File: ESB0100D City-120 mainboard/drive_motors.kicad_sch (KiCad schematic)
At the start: 47 parts, among them J1 Conn_01x02, J4 Conn_01x02, Q1 NPN, Q10 IRFZ44N, Q11 SPB18P06P, Q12 IRFZ44N, Q13 NPN, Q14 NPN, Q15 NPN, Q16 NPN, Q17 SPB18P06P, Q18 IRFZ44N, Q19 SPB18P06P, Q2 NPN, Q20 IRFZ44N, Q21 NPN, Q22 NPN, Q3 SPB18P06P, U10 74LS157, U11 74LS157, U4 74132

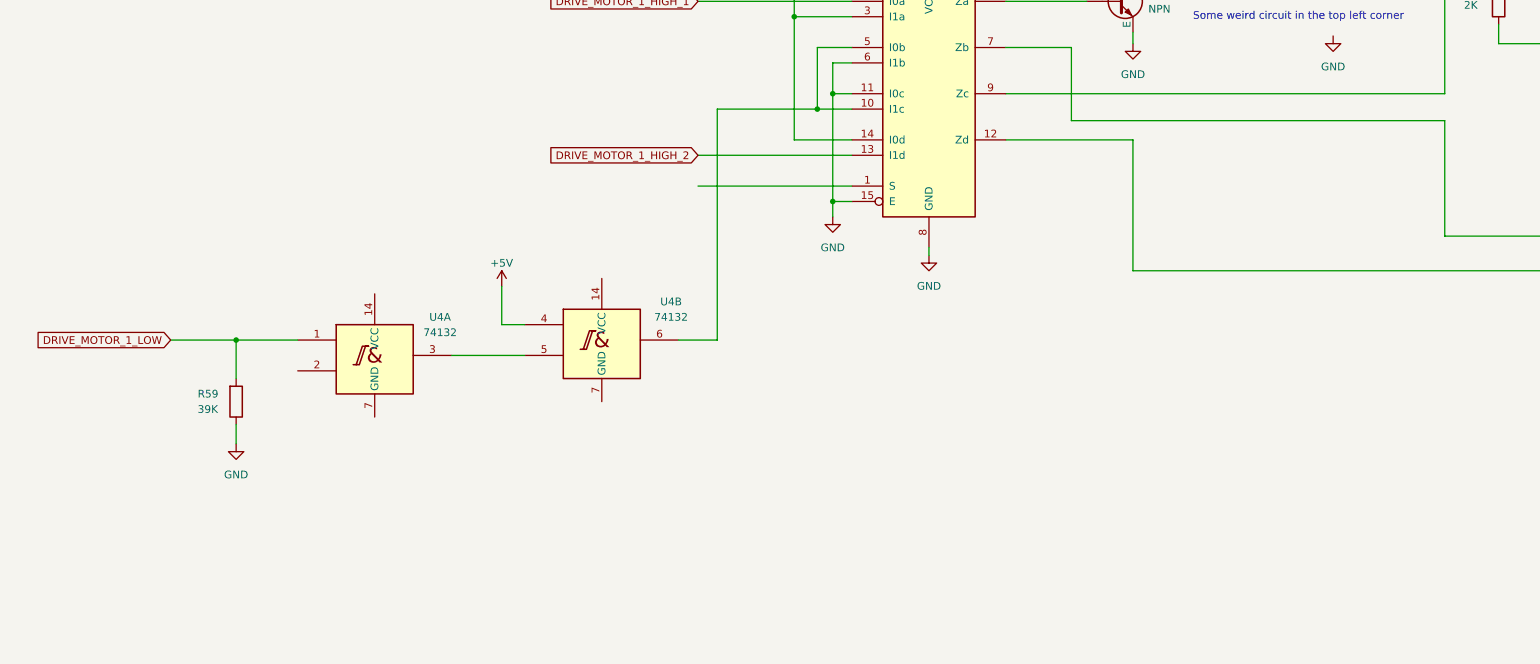
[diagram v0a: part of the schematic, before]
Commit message: Repo update
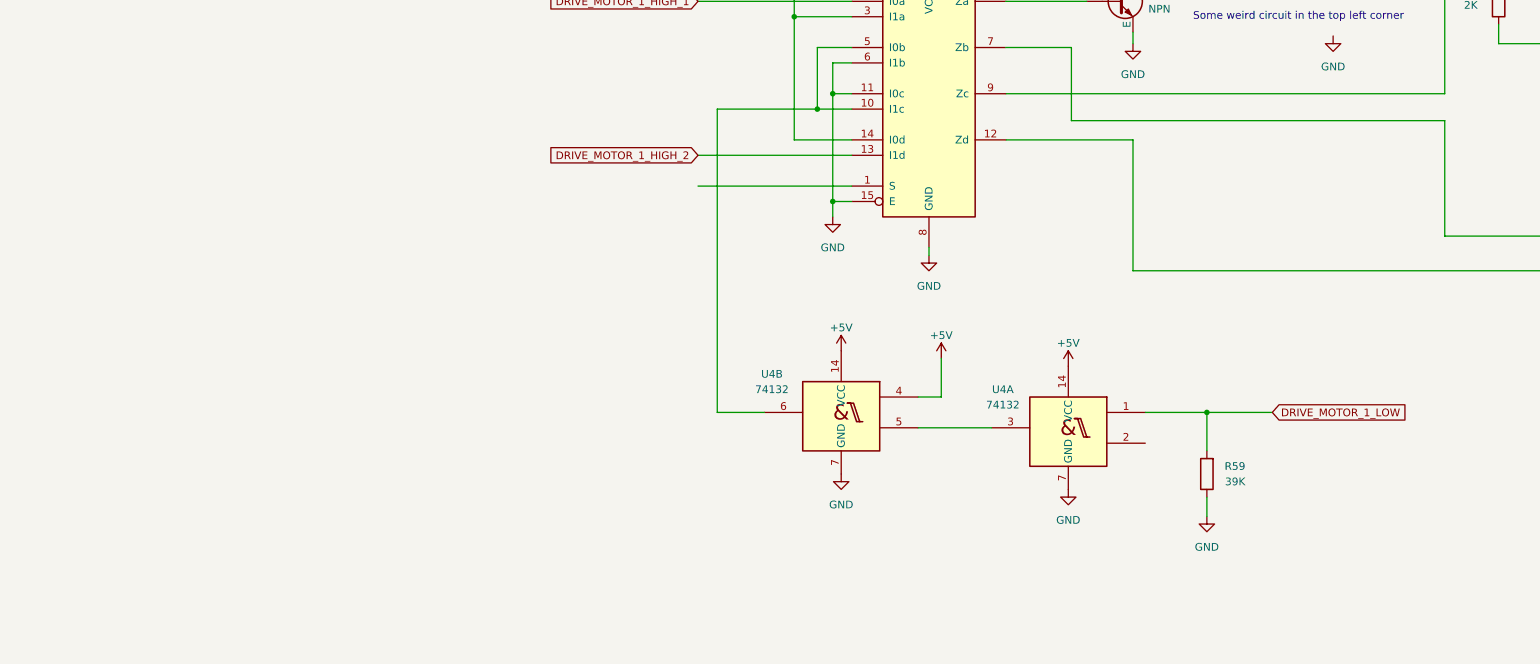
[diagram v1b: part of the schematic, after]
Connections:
- net +5V: now also U4.14 (VCC), U4.14 (VCC)
- net GND: now also U4.7 (GND), U4.7 (GND)
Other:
- moved on the sheet: R59, U4A, U4B
